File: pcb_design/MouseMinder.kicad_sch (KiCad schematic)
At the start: 23 parts, among them J3 Conn_02x04_Odd_Even, SW1 LCK-TA022H18-2WL, SW2 SKRPABE010, U1 PMS150C

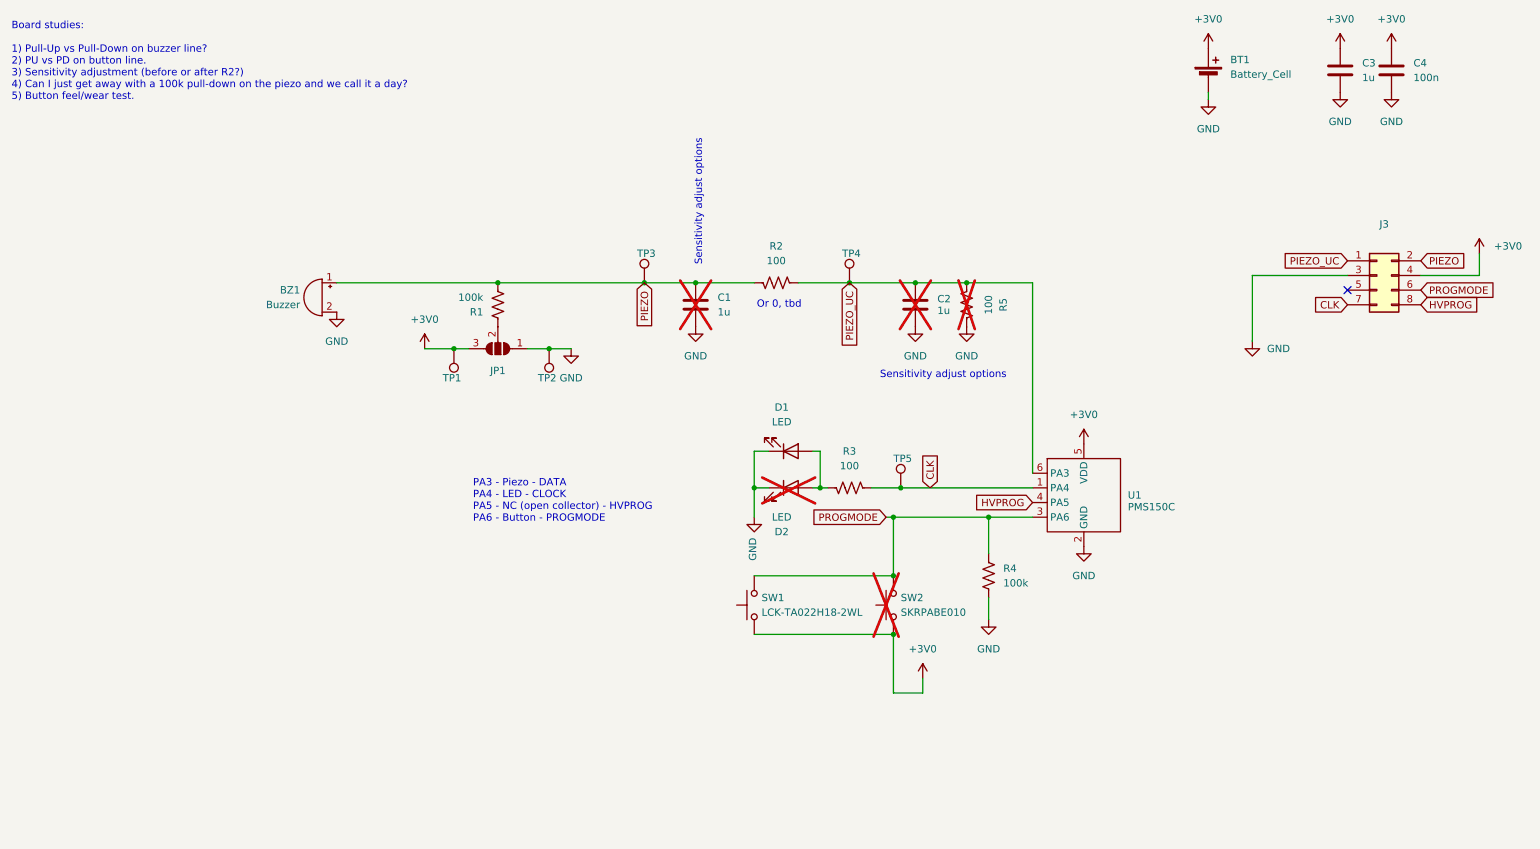
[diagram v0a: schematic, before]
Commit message: R6 sent to JLC Today. Here is the full prod snapshot.
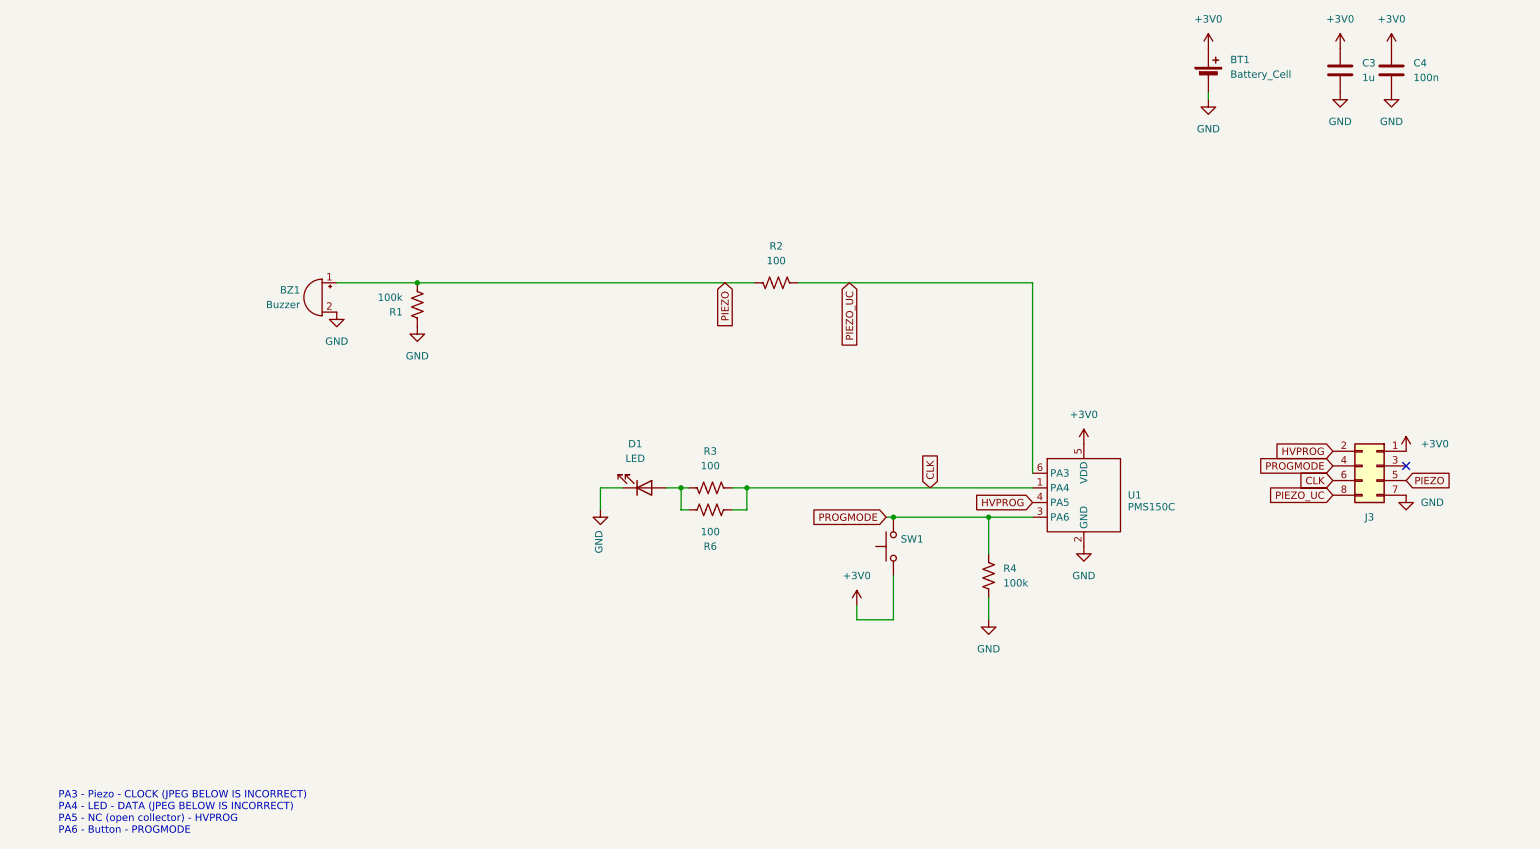
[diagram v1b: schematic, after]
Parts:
- removed C1, C2: 1u, Capacitor_SMD:C_0805_2012Metric, symbol Device:C
- removed D2: LED, LED_SMD:LED_0805_2012Metric, symbol Device:LED
- removed JP1: SolderJumper_3_Open, Jumper:SolderJumper-3_P1.3mm_Open_RoundedPad1.0x1.5mm_NumberLabels, symbol Jumper:SolderJumper_3_Open
- removed R5: 100, Resistor_SMD:R_0805_2012Metric, symbol Device:R_US
- removed SW2: SKRPABE010, 0conrads:SKRPABE010, symbol Switch:SW_Push
- removed TP1, TP2, TP3, TP4, TP5: TestPoint, TestPoint:TestPoint_Loop_D2.50mm_Drill1.0mm, symbol Connector:TestPoint
- added R6: 100, Resistor_SMD:R_0603_1608Metric, symbol Device:R_US
- BT1: footprint 0conrads:C70373 -> 0conrads:MY-2032-08; JLC_MPN C70373 -> C964832; MPN CR2032 3V -> C964832
- BZ1: MPN GSC1230YB-3V4000 -> C255333
- C3: footprint Capacitor_SMD:C_0805_2012Metric -> Capacitor_SMD:C_0603_1608Metric; JLC_MPN (none) -> C1592; MPN (none) -> C1592
- C4: footprint Capacitor_SMD:C_0805_2012Metric -> Capacitor_SMD:C_0603_1608Metric; JLC_MPN (none) -> C2909627; MPN (none) -> C2909627
- D1: MPN XL-2810UYC -> C3646949
- J3: footprint Connector_PinHeader_2.54mm:PinHeader_2x04_P2.54mm_Vertical -> 0conrads:2x8_POGO_CENTERING_HOLES
- R1, R4: footprint Resistor_SMD:R_0805_2012Metric -> Resistor_SMD:R_0603_1608Metric; JLC_MPN C25741 -> C25803; MPN 0402WGF1003TCE -> C25803
- R2, R3: footprint Resistor_SMD:R_0805_2012Metric -> Resistor_SMD:R_0603_1608Metric; JLC_MPN C25076 -> C2785067; MPN 0402WGF1000TCE -> C2785067
- SW1: MPN LCK-TA022H18-2WL -> C51978285
- U1: JLC_MPN (none) -> C168658; MPN (none) -> C168658
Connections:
- net +3V0: now also J3.1 (Pin_1); no longer J3.4 (Pin_4)
- net CLK: now also J3.6 (Pin_6), R6.1; no longer J3.7 (Pin_7)
- net GND: now also J3.7 (Pin_7), R1.1; no longer J3.3 (Pin_3)
- net HVPROG: now also J3.2 (Pin_2); no longer J3.8 (Pin_8)
- net PIEZO: now also J3.5 (Pin_5); no longer J3.2 (Pin_2)
- net PIEZO_UC: now also J3.8 (Pin_8); no longer J3.1 (Pin_1)
- net PROGMODE: now also J3.4 (Pin_4); no longer J3.6 (Pin_6)
- net at D1.2 (A), R3.2: now also R6.2
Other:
- note added: "PA3 - Piezo - CLOCK (JPEG BELOW IS INCORRECT) PA4 - LED - DATA (JPEG BELOW IS INCORRECT) PA5 - NC (open collector) - HVPROG PA6 - Button - PROGMODE"
- note removed: "Board studies: 1) Pull-Up vs Pull-Down on buzzer line? 2) PU vs PD on button line. 3) Sensitivity adjustment (before or after R2?) 4) Can I just get away with a 100k pull-down on the piezo and we call it a day? 5) Button feel/wear test."
- note removed: "Or 0, tbd"
- note removed: "PA3 - Piezo - DATA PA4 - LED - CLOCK PA5 - NC (open collector) - HVPROG PA6 - Button - PROGMODE"
- note removed: "Sensitivity adjust options"
- moved on the sheet: D1, J3, R1, R3, SW1

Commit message: Updated MPNs for tighter tolerance (100 ohms), older name-brand stock (caps), and tape-and-reel battery holder to reduce mfg cost
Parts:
- C4: JLC_MPN C2909627 -> C14663; MPN C2909627 -> C14663
- R2, R3, R6: JLC_MPN C2785067 -> C22775; MPN C2785067 -> C22775
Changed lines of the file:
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@@
 			)
 		)
-		(property "JLC_MPN" "C2909627"
+		(property "JLC_MPN" "C14663"
 			(at 256.54 26.67 0)
 			(effects
@@
 			)
 		)
-		(property "MPN" "C2909627"
+		(property "MPN" "C14663"
 			(at 256.54 26.67 0)
 			(effects
@@
 			)
 		)
-		(property "MPN" "C2785067"
+		(property "MPN" "C22775"
 			(at 149.86 63.5 90)
 			(effects
@@
 			)
 		)
-		(property "JLC_MPN" "C2785067"
+		(property "JLC_MPN" "C22775"
 			(at 149.86 63.5 90)
 			(effects
@@
 			)
 		)
-		(property "MPN" "C2785067"
+		(property "MPN" "C22775"
 			(at 138.43 102.87 90)
 			(effects
@@
 			)
 		)
-		(property "JLC_MPN" "C2785067"
+		(property "JLC_MPN" "C22775"
 			(at 138.43 102.87 90)
 			(effects
@@
 			)
 		)
-		(property "MPN" "C2785067"
+		(property "MPN" "C22775"
 			(at 138.43 99.06 90)
 			(effects
@@
 			)
 		)
-		(property "JLC_MPN" "C2785067"
+		(property "JLC_MPN" "C22775"
 			(at 138.43 99.06 90)
 			(effects
